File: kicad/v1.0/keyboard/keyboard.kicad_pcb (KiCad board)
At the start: 2 copper layers, 145 x 71.6 mm, 101 parts, among them J1 PMOD, J10 Cassette Input, J11 Cassette Output, J12 SD_Card, J2 Conn_01x02, J3 Conn_01x02, J4 Interface Connector, J5 Programmer, J9 SD_Card, SW1 @, SW10 I, SW11 J, SW12 K, SW13 L, SW14 M, SW15 N, SW16 O, SW17 P, SW18 Q, SW19 R, SW2 A, SW20 S, SW21 T, SW22 U, SW23 V, SW24 W, SW25 X, SW26 Y, SW27 Z, SW28 0, SW29 1, SW3 B, SW30 2, SW31 3, SW32 4, SW33 5, SW34 6, SW35 7, SW36 0, SW37 1, SW38 2, SW39 3, SW4 C, SW40 4, SW41 5, SW42 6, SW43 7, SW44 8, SW45 9, SW46 ., SW47 8, SW48 9, SW49 :, SW5 D, SW50 ;, SW51 ,, SW52 -, SW53 ., SW54 /, SW55 ENTER, SW56 ENTER, SW57 CLEAR, SW58 BREAK, SW59 UP, SW6 E, SW60 DOWN, SW61 LEFT, SW62 RIGHT, SW63 SPACE, SW64 RESET, SW65 RSHIFT, SW66 LSHIFT, SW67 SPACE, SW68 SPACE, SW69 ENTER, SW7 F, SW70 ESP_RESET, SW71 PTRS_RESET, SW72 TRS_IO_STATUS, SW8 G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

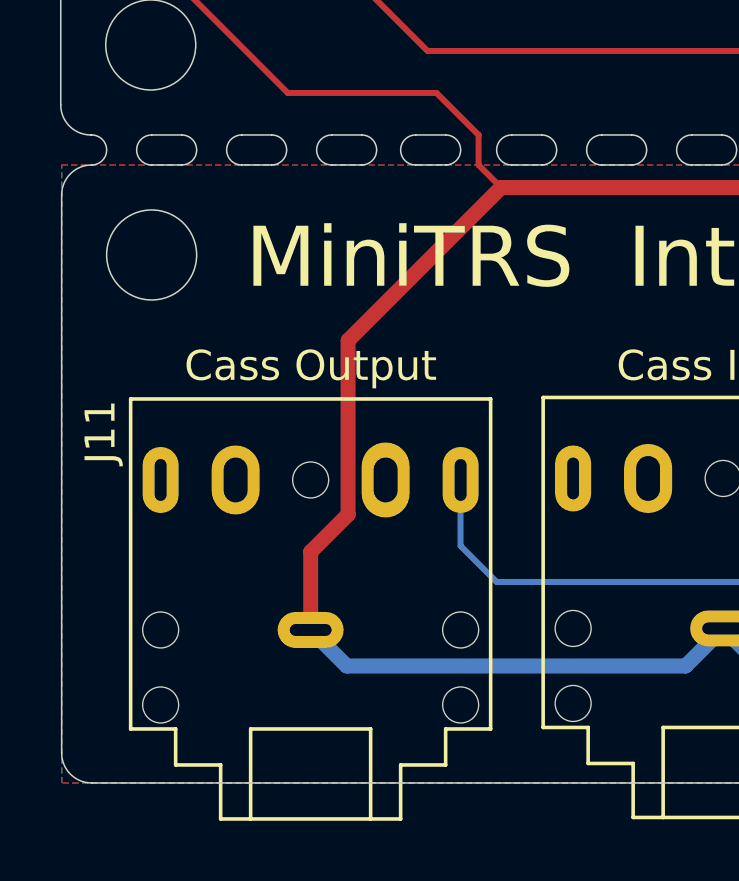
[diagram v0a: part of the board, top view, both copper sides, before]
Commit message: Update keyboard.kicad_pcb
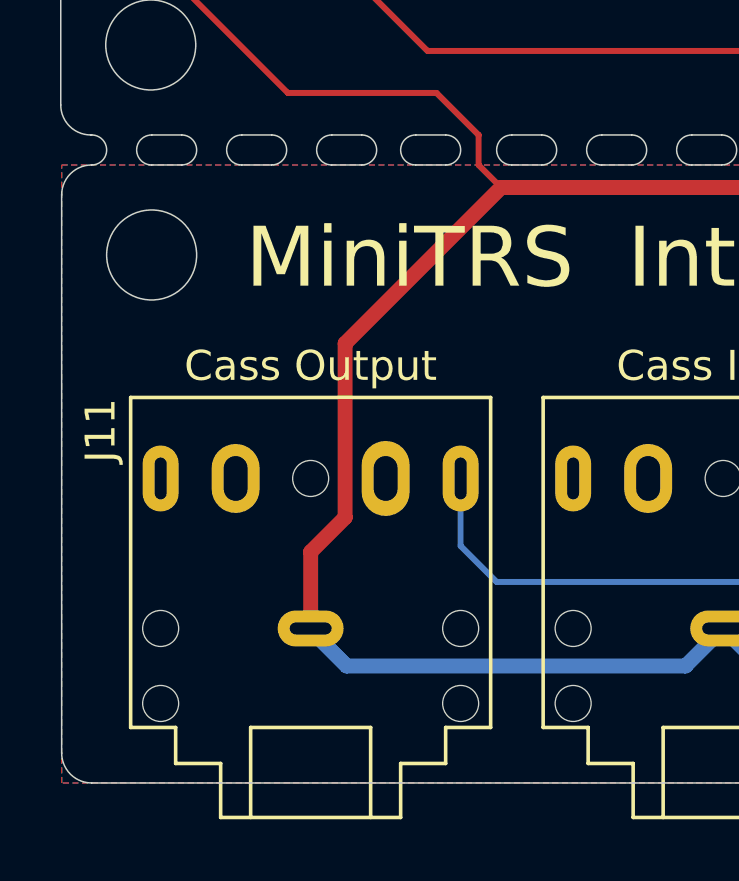
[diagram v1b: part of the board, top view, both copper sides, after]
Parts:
- moved J11 0.05 mm to (77.6, 139.9)
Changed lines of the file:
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@@
 	(footprint "Connector_Audio:Jack_3.5mm_CUI_SJ1-3525N_Horizontal"
 		(layer "F.Cu")
-		(at 77.6 140)
+		(at 77.6 139.95)
 		(descr "TRS 3.5mm, horizontal, through-hole, https://www.cuidevices.com/product/resource/pdf/sj1-352xn.pdf")
 		(tags "TRS audio jack stereo horizontal")
@@
 	)
 	(segment
+		(start 77.6 139.95)
+		(end 77.6 137.4)
+		(width 0.5)
+		(layer "F.Cu")
+		(net 3)
+	)
+	(segment
 		(start 180.9 137.3)
 		(end 185.1 137.3)
@@
 	)
 	(segment
-		(start 77.6 137.4)
-		(end 78.849 136.151)
-		(width 0.5)
-		(layer "F.Cu")
-		(net 3)
-	)
-	(segment
 		(start 83.2 124.502)
 		(end 83.949 125.251)
@@
 	)
 	(segment
-		(start 78.849 136.151)
-		(end 78.849 130.351)
-		(width 0.5)
-		(layer "F.Cu")
-		(net 3)
-	)
-	(segment
 		(start 109.85 137.75)
 		(end 109.9 137.7)
@@
 	)
 	(segment
+		(start 78.75 136.25)
+		(end 78.75 130.45)
+		(width 0.5)
+		(layer "F.Cu")
+		(net 3)
+	)
+	(segment
 		(start 137.6 143.8)
 		(end 143.95 143.8)
@@
 	)
 	(segment
-		(start 78.849 130.351)
-		(end 83.949 125.251)
-		(width 0.5)
-		(layer "F.Cu")
-		(net 3)
-	)
-	(segment
 		(start 110.2 127.1)
 		(end 114 127.1)
@@
 	)
 	(segment
-		(start 77.6 140)
-		(end 77.6 137.4)
-		(width 0.5)
-		(layer "F.Cu")
-		(net 3)
-	)
-	(segment
 		(start 78.84 81.1)
 		(end 72.7 81.1)
@@
 	)
 	(segment
+		(start 77.6 137.4)
+		(end 78.75 136.25)
+		(width 0.5)
+		(layer "F.Cu")
+		(net 3)
+	)
+	(segment
 		(start 169.71 143.7)
 		(end 176 143.7)
@@
 	)
 	(segment
+		(start 78.75 130.45)
+		(end 83.949 125.251)
+		(width 0.5)
+		(layer "F.Cu")
+		(net 3)
+	)
+	(segment
 		(start 137.6 143.8)
 		(end 128.4 143.8)
@@
 	)
 	(segment
+		(start 78.8 141.2)
+		(end 90.1 141.2)
+		(width 0.5)
+		(layer "B.Cu")
+		(net 3)
+	)
+	(segment
 		(start 114.33 80.500001)
 		(end 113.867499 80.0375)
@@
 	)
 	(segment
-		(start 90.1 141.2)
-		(end 91.35 139.95)
-		(width 0.5)
-		(layer "B.Cu")
-		(net 3)
-	)
-	(segment
 		(start 109.47 80.0375)
 		(end 109.47 81.47)
@@
 	)
 	(segment
+		(start 90.1 141.2)
+		(end 91.35 139.95)
+		(width 0.5)
+		(layer "B.Cu")
+		(net 3)
+	)
+	(segment
 		(start 78.97 81.23)
 		(end 78.97 80.0375)
@@
 	)
 	(segment
-		(start 78.8 141.2)
-		(end 90.1 141.2)
+		(start 77.6 139.95)
+		(end 77.6 140)
 		(width 0.5)
 		(layer "B.Cu")
@@
 	)
 	(segment
-		(start 77.6 140)
-		(end 78.8 141.2)
-		(width 0.5)
-		(layer "B.Cu")
-		(net 3)
-	)
-	(segment
 		(start 113.062499 80.0375)
 		(end 111.8 80.0375)
@@
 		(layer "B.Cu")
 		(net 3)
+	)
+	(segment
+		(start 77.6 140)
+		(end 78.8 141.2)
+		(width 0.5)
+		(layer "B.Cu")
+		(net 3)
